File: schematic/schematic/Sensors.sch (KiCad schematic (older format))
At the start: 13 parts, among them U10 MPU-9250, U11 MPU-9250, U9 INA219AIDCNR

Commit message: assign footprint
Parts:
- C22, C29, C30, C32, C33: footprint (none) -> micelib:C_0402_1005Metric_HandSoldering
- C28, C31: footprint (none) -> micelib:C_0201_0603Metric_HandSoldering
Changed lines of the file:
@@
 F 0 "C22" H 1550 1350 50  0000 L CNN
 F 1 "0.1u" H 1550 1250 50  0000 L CNN
-F 2 "" H 1450 1300 50  0001 C CNN
+F 2 "micelib:C_0402_1005Metric_HandSoldering" H 1450 1300 50  0001 C CNN
 F 3 "~" H 1450 1300 50  0001 C CNN
 	1    1450 1300
@@
 F 0 "C30" V 3471 4500 50  0000 C CNN
 F 1 "0.1u" V 3562 4500 50  0000 C CNN
-F 2 "" H 3700 4500 50  0001 C CNN
+F 2 "micelib:C_0402_1005Metric_HandSoldering" H 3700 4500 50  0001 C CNN
 F 3 "~" H 3700 4500 50  0001 C CNN
 	1    3700 4500
@@
 F 0 "C33" V 6271 4500 50  0000 C CNN
 F 1 "0.1u" V 6362 4500 50  0000 C CNN
-F 2 "" H 6500 4500 50  0001 C CNN
+F 2 "micelib:C_0402_1005Metric_HandSoldering" H 6500 4500 50  0001 C CNN
 F 3 "~" H 6500 4500 50  0001 C CNN
 	1    6500 4500
@@
 F 0 "C28" H 1742 3496 50  0000 L CNN
 F 1 "10n" H 1742 3405 50  0000 L CNN
-F 2 "" H 1650 3450 50  0001 C CNN
+F 2 "micelib:C_0201_0603Metric_HandSoldering" H 1650 3450 50  0001 C CNN
 F 3 "~" H 1650 3450 50  0001 C CNN
 	1    1650 3450
@@
 F 0 "C29" H 2092 3496 50  0000 L CNN
 F 1 "0.1u" H 2092 3405 50  0000 L CNN
-F 2 "" H 2000 3450 50  0001 C CNN
+F 2 "micelib:C_0402_1005Metric_HandSoldering" H 2000 3450 50  0001 C CNN
 F 3 "~" H 2000 3450 50  0001 C CNN
 	1    2000 3450
@@
 F 0 "C31" H 4542 3496 50  0000 L CNN
 F 1 "10n" H 4542 3405 50  0000 L CNN
-F 2 "" H 4450 3450 50  0001 C CNN
+F 2 "micelib:C_0201_0603Metric_HandSoldering" H 4450 3450 50  0001 C CNN
 F 3 "~" H 4450 3450 50  0001 C CNN
 	1    4450 3450
@@
 F 0 "C32" H 4892 3496 50  0000 L CNN
 F 1 "0.1u" H 4892 3405 50  0000 L CNN
-F 2 "" H 4800 3450 50  0001 C CNN
+F 2 "micelib:C_0402_1005Metric_HandSoldering" H 4800 3450 50  0001 C CNN
 F 3 "~" H 4800 3450 50  0001 C CNN
 	1    4800 3450

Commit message: wip: add another layer
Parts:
- R11, R27, R28: footprint (none) -> micelib:C_0402_1005Metric_HandSoldering
- U10, U11: footprint Sensor_Motion:InvenSense_QFN-24_3x3mm_P0.4mm -> micelib:InvenSense_QFN-24_3x3mm_P0.4mm_HandSoldering
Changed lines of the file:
@@
 F 0 "R27" V 1200 1150 50  0000 C CNN
 F 1 "10" V 1400 1150 50  0000 C CNN
-F 2 "" H 1300 1150 50  0001 C CNN
+F 2 "micelib:C_0402_1005Metric_HandSoldering" H 1300 1150 50  0001 C CNN
 F 3 "~" H 1300 1150 50  0001 C CNN
 	1    1300 1150
@@
 F 0 "R28" V 1200 1450 50  0000 C CNN
 F 1 "10" V 1400 1450 50  0000 C CNN
-F 2 "" H 1300 1450 50  0001 C CNN
+F 2 "micelib:C_0402_1005Metric_HandSoldering" H 1300 1450 50  0001 C CNN
 F 3 "~" H 1300 1450 50  0001 C CNN
 	1    1300 1450
@@
 F 0 "R11" H 1300 1250 50  0000 C CNN
 F 1 "2m" H 1250 1350 50  0000 C CNN
-F 2 "" H 1150 1300 50  0001 C CNN
+F 2 "micelib:C_0402_1005Metric_HandSoldering" H 1150 1300 50  0001 C CNN
 F 3 "~" H 1150 1300 50  0001 C CNN
 	1    1150 1300
@@
 F 0 "U10" H 2850 4300 50  0000 C CNN
 F 1 "MPU-9250" H 2850 4200 50  0000 C CNN
-F 2 "Sensor_Motion:InvenSense_QFN-24_3x3mm_P0.4mm" H 2850 3300 50  0001 C CNN
+F 2 "micelib:InvenSense_QFN-24_3x3mm_P0.4mm_HandSoldering" H 2850 3300 50  0001 C CNN
 F 3 "https://store.invensense.com/datasheets/invensense/MPU9250REV1.0.pdf" H 2850 4150 50  0001 C CNN
 	1    2850 4300
@@
 F 0 "U11" H 5650 4300 50  0000 C CNN
 F 1 "MPU-9250" H 5650 4200 50  0000 C CNN
-F 2 "Sensor_Motion:InvenSense_QFN-24_3x3mm_P0.4mm" H 5650 3300 50  0001 C CNN
+F 2 "micelib:InvenSense_QFN-24_3x3mm_P0.4mm_HandSoldering" H 5650 3300 50  0001 C CNN
 F 3 "https://store.invensense.com/datasheets/invensense/MPU9250REV1.0.pdf" H 5650 4150 50  0001 C CNN
 	1    5650 4300

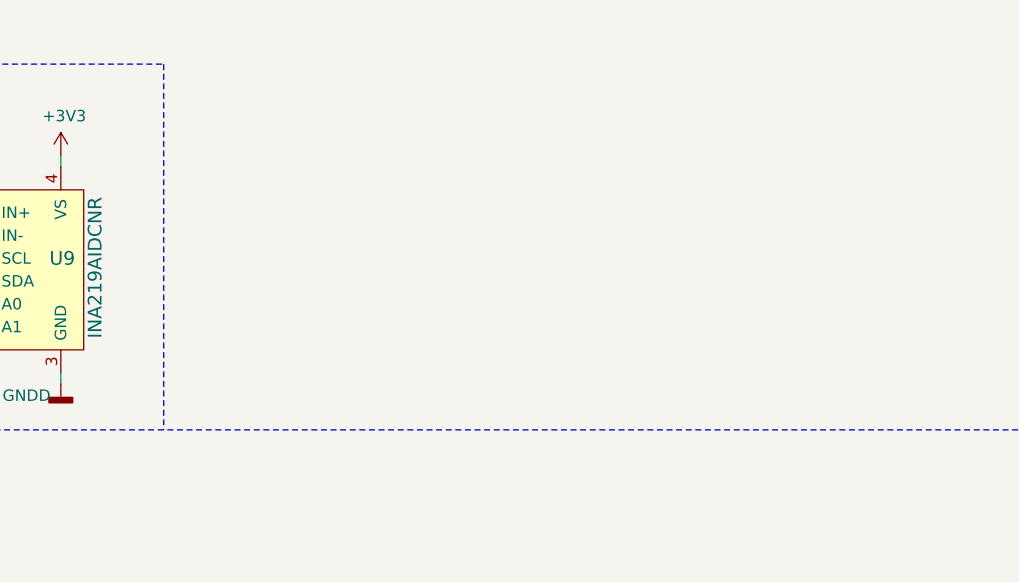
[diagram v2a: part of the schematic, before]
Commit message: 配置開始
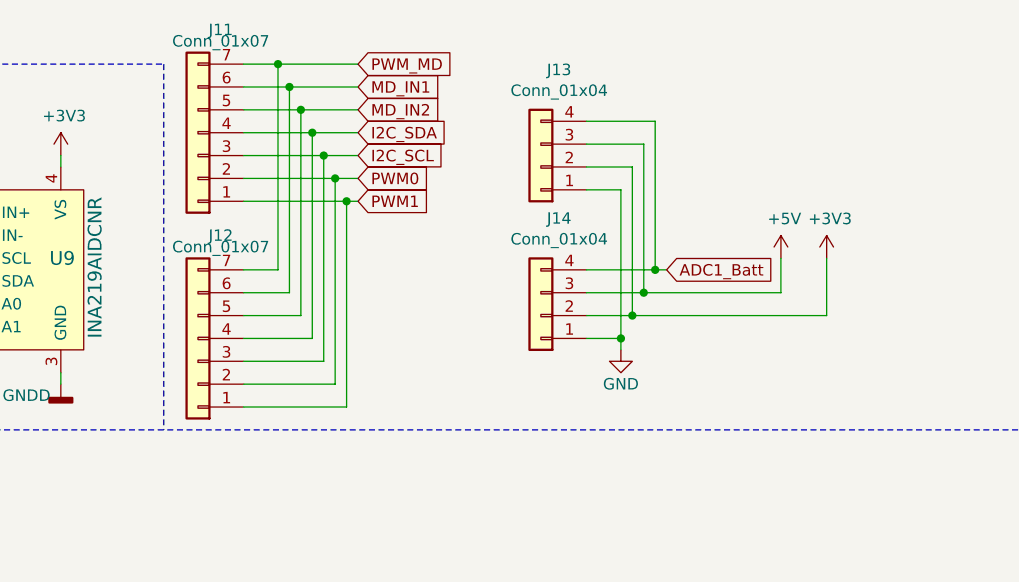
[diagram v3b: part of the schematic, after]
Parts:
- added J11, J12: Conn_01x07, Connector_PinSocket_2.54mm:PinSocket_1x07_P2.54mm_Vertical, symbol Connector_Generic:Conn_01x07
- added J13, J14: Conn_01x04, Connector_PinSocket_2.54mm:PinSocket_1x04_P2.54mm_Vertical, symbol Connector_Generic:Conn_01x04
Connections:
- net +3V3: now also J13.2 (Pin_2), J14.2 (Pin_2)
- net +5V: now also J13.3 (Pin_3), J14.3 (Pin_3)
- net I2C_SCL: now also J11.3 (Pin_3), J12.3 (Pin_3)
- net I2C_SDA: now also J11.4 (Pin_4), J12.4 (Pin_4)
- new net ADC1_Batt: J13.4 (Pin_4), J14.4 (Pin_4)
- new net GND: J13.1 (Pin_1), J14.1 (Pin_1)
- new net MD_IN1: J11.6 (Pin_6), J12.6 (Pin_6)
- new net MD_IN2: J11.5 (Pin_5), J12.5 (Pin_5)
- new net PWM0: J11.2 (Pin_2), J12.2 (Pin_2)
- new net PWM1: J11.1 (Pin_1), J12.1 (Pin_1)
- new net PWM_MD: J11.7 (Pin_7), J12.7 (Pin_7)
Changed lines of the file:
@@
 Wire Notes Line
 	6800 6450 600  6450
+Text GLabel 3500 700  2    50   Input ~ 0
+PWM_MD
+Text GLabel 3500 800  2    50   Input ~ 0
+MD_IN1
+Text GLabel 3500 900  2    50   Input ~ 0
+MD_IN2
+Text GLabel 3500 1000 2    50   Input ~ 0
+I2C_SDA
+Text GLabel 3500 1100 2    50   Input ~ 0
+I2C_SCL
+$Comp
+L power:GND #PWR?
+U 1 1 5EC61195
+P 4650 1950
+AR Path="/5EC61195" Ref="#PWR?"  Part="1"
+AR Path="/5E247314/5EC61195" Ref="#PWR075"  Part="1"
+F 0 "#PWR075" H 4650 1700 50  0001 C CNN
+F 1 "GND" H 4650 1800 50  0000 C CNN
+F 2 "" H 4650 1950 50  0001 C CNN
+F 3 "" H 4650 1950 50  0001 C CNN
+	1    4650 1950
+	1    0    0    -1
+$EndComp
+Text GLabel 4850 1600 2    50   Input ~ 0
+ADC1_Batt
+Wire Wire Line
+	4650 1950 4650 1900
+$Comp
+L Connector_Generic:Conn_01x04 J14
+U 1 1 5ECB2FF3
+P 4300 1800
+F 0 "J14" H 4220 1375 50  0000 C CNN
+F 1 "Conn_01x04" H 4220 1466 50  0000 C CNN
+F 2 "Connector_PinSocket_2.54mm:PinSocket_1x04_P2.54mm_Vertical" H 4300 1800 50  0001 C CNN
+F 3 "~" H 4300 1800 50  0001 C CNN
+	1    4300 1800
+	-1   0    0    1
+$EndComp
+$Comp
+L Connector_Generic:Conn_01x04 J13
+U 1 1 5ECB3055
+P 4300 1150
+F 0 "J13" H 4220 725 50  0000 C CNN
+F 1 "Conn_01x04" H 4220 816 50  0000 C CNN
+F 2 "Connector_PinSocket_2.54mm:PinSocket_1x04_P2.54mm_Vertical" H 4300 1150 50  0001 C CNN
+F 3 "~" H 4300 1150 50  0001 C CNN
+	1    4300 1150
+	-1   0    0    1
+$EndComp
+Wire Wire Line
+	4500 1900 4650 1900
+$Comp
+L power:+3V3 #PWR077
+U 1 1 5ECBE3B6
+P 5550 1550
+F 0 "#PWR077" H 5550 1400 50  0001 C CNN
+F 1 "+3V3" H 5565 1723 50  0000 C CNN
+F 2 "" H 5550 1550 50  0001 C CNN
+F 3 "" H 5550 1550 50  0001 C CNN
+	1    5550 1550
+	1    0    0    -1
+$EndComp
+$Comp
+L power:+5V #PWR076
+U 1 1 5ECBE416
+P 5350 1550
+F 0 "#PWR076" H 5350 1400 50  0001 C CNN
+F 1 "+5V" H 5365 1723 50  0000 C CNN
+F 2 "" H 5350 1550 50  0001 C CNN
+F 3 "" H 5350 1550 50  0001 C CNN
+	1    5350 1550
+	1    0    0    -1
+$EndComp
+Wire Wire Line
+	5350 1550 5350 1700
+Wire Wire Line
+	4650 1900 4650 1250
+Wire Wire Line
+	4650 1250 4500 1250
+Connection ~ 4650 1900
+Wire Wire Line
+	4500 1700 4750 1700
+Wire Wire Line
+	4500 1800 4700 1800
+Wire Wire Line
+	4500 1150 4700 1150
+Wire Wire Line
+	4700 1150 4700 1800
+Connection ~ 4700 1800
+Wire Wire Line
+	4500 1050 4750 1050
+Wire Wire Line
+	4750 1050 4750 1700
+Connection ~ 4750 1700
+Wire Wire Line
+	5550 1550 5550 1800
+Wire Wire Line
+	4750 1700 5350 1700
+Wire Wire Line
+	4700 1800 5550 1800
+Wire Wire Line
+	4500 950  4800 950
+Wire Wire Line
+	4800 950  4800 1600
+Wire Wire Line
+	4800 1600 4500 1600
+Wire Wire Line
+	4850 1600 4800 1600
+Connection ~ 4800 1600
+Text GLabel 3500 1200 2    50   Input ~ 0
+PWM0
+Text GLabel 3500 1300 2    50   Input ~ 0
+PWM1
+$Comp
+L Connector_Generic:Conn_01x07 J11
+U 1 1 5ED4250E
+P 2800 1000
+F 0 "J11" H 2700 550 50  0000 C CNN
+F 1 "Conn_01x07" H 2700 600 50  0000 C CNN
+F 2 "Connector_PinSocket_2.54mm:PinSocket_1x07_P2.54mm_Vertical" H 2800 1000 50  0001 C CNN
+F 3 "~" H 2800 1000 50  0001 C CNN
+	1    2800 1000
+	-1   0    0    1
+$EndComp
+$Comp
+L Connector_Generic:Conn_01x07 J12
+U 1 1 5ED425C0
+P 2800 1900
+F 0 "J12" H 2700 1450 50  0000 C CNN
+F 1 "Conn_01x07" H 2700 1500 50  0000 C CNN
+F 2 "Connector_PinSocket_2.54mm:PinSocket_1x07_P2.54mm_Vertical" H 2800 1900 50  0001 C CNN
+F 3 "~" H 2800 1900 50  0001 C CNN
+	1    2800 1900
+	-1   0    0    1
+$EndComp
+Wire Wire Line
+	3000 700  3150 700
+Wire Wire Line
+	3000 800  3200 800
+Wire Wire Line
+	3000 900  3250 900
+Wire Wire Line
+	3000 1000 3300 1000
+Wire Wire Line
+	3000 1100 3350 1100
+Wire Wire Line
+	3000 1200 3400 1200
+Wire Wire Line
+	3000 1600 3150 1600
+Wire Wire Line
+	3150 1600 3150 700
+Connection ~ 3150 700
+Wire Wire Line
+	3200 1700 3000 1700
+Wire Wire Line
+	3000 1800 3250 1800
+Wire Wire Line
+	3250 1800 3250 900
+Connection ~ 3250 900
+Wire Wire Line
+	3200 1700 3200 800
+Connection ~ 3200 800
+Wire Wire Line
+	3300 1000 3300 1900
+Wire Wire Line
+	3300 1900 3000 1900
+Connection ~ 3300 1000
+Wire Wire Line
+	3000 2000 3350 2000
+Wire Wire Line
+	3350 2000 3350 1100
+Connection ~ 3350 1100
+Wire Wire Line
+	3400 1200 3400 2100
+Wire Wire Line
+	3400 2100 3000 2100
+Connection ~ 3400 1200
+Wire Wire Line
+	3000 1300 3450 1300
+Wire Wire Line
+	3400 1200 3500 1200
+Wire Wire Line
+	3350 1100 3500 1100
+Wire Wire Line
+	3300 1000 3500 1000
+Wire Wire Line
+	3250 900  3500 900
+Wire Wire Line
+	3200 800  3500 800
+Wire Wire Line
+	3150 700  3500 700
+Wire Wire Line
+	3450 1300 3450 2200
+Wire Wire Line
+	3450 2200 3000 2200
 Wire Bus Line
 	1550 5550 1550 5950
@@
 Wire Bus Line
 	4000 3100 4000 4100
+Connection ~ 3450 1300
+Wire Wire Line
+	3450 1300 3500 1300
 $EndSCHEMATC
